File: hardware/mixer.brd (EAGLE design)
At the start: 113.2 x 100 mm, 199 parts, among them IC1 PGA2311, IC10 OPA2134P, IC11 OPA2134P, IC12 OPA2134P, IC13 OPA2134P, IC2 PGA2311, IC3 PGA2311, IC4 PGA2311, IC5 PGA2311, IC6 OPA2134P, IC7 OPA2134P, IC8 OPA2134P, IC9 OPA2134P, Q1 SI2305, Q2 MOSFET-NCHANNEL_SOT23-3, X1 MOLEX_6HORIZONTAL, X2 MOLEX_6HORIZONTAL, X3 MOLEX_4HORIZONTAL, Y1 32768Hz CFPX-217 12.5pF

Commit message: routing
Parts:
- removed C47, C51, C52: 100n, rcl:C0805
- removed C64, C65, C66, C67, C68, C69, C71, C72, C73, C74, C75, C76, C78, C88, C89, C90: 10u, rcl:153CLV-0405
- removed R92, R93, R94, R95: 0R_0805, Simplex-Jumpers:R0805W
- removed U$10, U$3, U$4, U$8: RESETTABLE, Simplex-Fuses:1210
- added C17, C18, C19, C20, C21, C22, C24, C25, C26, C28, C32, C33, C63, C79, C80: 100n, rcl:C0805
- added C92, C96: 10u, rcl:153CLV-0405
- added R96, R97: 0R_0805, Simplex-Jumpers:R0805W
- added R98, R99: DNP, rcl:R0805W
- added U$12, U$13, U$2, U$5, U$6, U$9: RESETTABLE, Simplex-Fuses:1210
- added X4: inputs, con-3m:PAK100/2500-14
- added X5: outputs, con-3m:PAK100/2500-14
- X2: value MOLEX_6HORIZONTAL -> 2514-; device Simplex-Connectors:0530480610 -> con-3m:PAK100/2500-14
- X3: value MOLEX_4HORIZONTAL -> display
- moved C87 813.4 mm to (4.60, 60.5)
- moved C58 769.7 mm to (38.5, 89.5), flipped to the bottom, turned to 270 degrees
- moved C91 767.9 mm to (19.4, 3.60)
- moved C59 753.2 mm to (38.5, 70.5), flipped to the bottom, turned to 270 degrees
- moved C60 737.8 mm to (38.6, 52.2), flipped to the bottom, turned to 270 degrees
- moved C61 722.1 mm to (38.6, 33.6), flipped to the bottom, turned to 270 degrees
- moved C62 705.7 mm to (38.6, 14.2), flipped to the bottom, turned to 270 degrees
- moved LED2 661.9 mm to (12.4, 54.8)
- moved R33 661.9 mm to (23.4, 59.5)
- moved C45 631.9 mm to (22.4, 90.2), turned to 180 degrees
- moved C84 630.1 mm to (10.4, 59.6)
- moved C85 630.1 mm to (14.4, 59.6)
- moved C86 630.1 mm to (6.40, 53.5)
- moved C50 612.5 mm to (22.4, 71.0), turned to 180 degrees
- moved C81 608.1 mm to (22.4, 52.9), turned to 180 degrees
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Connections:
- removed net +3V: C84.1, C85.1, C86.1, C87.+, R95.2
- removed net +5V_DIG: Q1.2, R37.2, R92.1
- removed net A+5V: C29.1, C30.1, C31.1, C34.1, C35.1, C36.1, C37.1, C46.1, C47.1, C48.1, C49.1, C58.2, C59.2, C60.2, C61.2, C62.2, C64.+, C65.+, C66.+, C67.+, C68.+, C69.+, C70.+, IC1.12, IC10.8, IC11.8, IC12.8, IC13.8, IC2.12, IC3.12, IC4.12, IC5.12, IC6.8, IC7.8, IC8.8, IC9.8, R94.1
- removed net A-5V: C38.1, C39.1, C40.1, C41.1, C42.1, C43.1, C44.1, C51.1, C52.1, C53.1, C54.1, C58.1, C59.1, C60.1, C61.1, C62.1, C71.-, C72.-, C73.-, C74.-, C75.-, C76.-, C77.-, IC1.13, IC10.4, IC11.4, IC12.4, IC13.4, IC2.13, IC3.13, IC4.13, IC5.13, IC6.4, IC7.4, IC8.4, IC9.4, R93.1
- removed net N$24: U$4.P$2, X2.4
- removed net N$25: U$8.P$2, X2.3
- removed net N$3: R92.2, U$8.P$1
- removed net N$34: U$10.P$2, X2.2
- removed net N$6: R95.1, U$10.P$1
- removed net N$60: R94.2, U$3.P$1
- removed net N$62: R93.2, U$4.P$1
- removed net N$63: U$3.P$2, X2.5
- removed net VCC: R34.2, U$11.11, U$11.28, U$11.7, X1.4
- new net +15V: C17.1, C18.1, C24.1, C25.1, C33.1, C63.1, C79.1, C80.1, C92.+, IC10.8, IC11.8, IC12.8, IC13.8, U$2.P$2
- new net +5V: C26.2, C28.2, C29.1, C30.1, C31.1, C32.2, C34.1, C35.1, C36.1, C37.1, C46.2, C48.1, C49.1, C58.2, C59.2, C60.2, C61.2, C62.2, C70.+, IC1.12, IC2.12, IC3.12, IC4.12, IC5.12, IC6.8, IC7.8, IC8.8, IC9.8, U$6.P$2
- new net +5V/1: Q1.2, R37.2, U$12.P$2
- new net -15V: C19.1, C20.1, C21.1, C22.1, C33.2, C63.2, C79.2, C80.2, C96.+, IC10.4, IC11.4, IC12.4, IC13.4, U$5.P$2
- new net -5V: C26.1, C28.1, C32.1, C38.1, C39.1, C40.1, C41.1, C42.1, C43.1, C44.1, C46.1, C53.1, C54.1, C58.1, C59.1, C60.1, C61.1, C62.1, C77.-, IC1.13, IC2.13, IC3.13, IC4.13, IC5.13, IC6.4, IC7.4, IC8.4, IC9.4, U$9.P$2
- new net 3V3: C84.1, C85.1, C86.1, C87.+, R34.2, U$11.11, U$11.28, U$11.7, U$13.P$2, X1.4, X3.1
- new net N$79: IC5.9, R97.1, R99.2
- new net N$80: JP2.2, R97.2
- new net N$85: U$2.P$1, X2.12
- new net N$86: U$5.P$1, X2.10
- new net N$88: U$6.P$1, X2.8
- new net N$89: U$9.P$1, X2.6
- new net N$90: U$12.P$1, X2.4
- new net N$91: U$13.P$1, X2.2
- net +5V_PGA: no longer C78.+, C88.+, C89.+, C90.+
- net AGND: now also C17.2, C18.2, C19.2, C20.2, C21.2, C22.2, C24.2, C25.2, C92.-, C96.-, R98.1, R99.1, X2.11, X2.13, X2.7, X2.9, X4.1, X4.10, X4.13, X4.4, X4.7, X5.10, X5.12, X5.14, X5.2, X5.4, X5.6, X5.8; no longer C46.2, C47.2, C51.2, C52.2, C64.-, C65.-, C66.-, C67.-, C68.-, C69.-, C71.+, C72.+, C73.+, C74.+, C75.+, C76.+, X2.6
- net DGND: now also X2.3, X2.5; no longer C78.-, C88.-, C89.-, C90.-, X3.1
- net FRONT_L: now also X4.2
- net FRONT_R: now also X4.3
- net LINE_L: now also X4.5
- net LINE_R: now also X4.6
- net M_FRONT_L: now also X5.11
- net M_FRONT_R: now also X5.13
- net M_REAR_L: now also X5.7
- net M_REAR_R: now also X5.9
- net N$36: now also R96.2; no longer IC5.16
- net N$42: now also IC5.16, R96.1, R98.2; no longer IC5.9, JP2.2
- net REAR_L: now also X4.11
- net REAR_R: now also X4.12
- net SPDIF_L: now also X4.8
- net SPDIF_R: now also X4.9
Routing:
- net +5V: track 0.00 -> 259.3 mm, vias 0 -> 9
- net -5V: track 0.00 -> 256.0 mm, vias 0 -> 16
- net +5V_PGA: track 0.00 -> 135.9 mm, vias 0 -> 5
- net AGND: track 26.3 -> 148.1 mm, vias 13 -> 53
- net +15V: track 0.00 -> 102.7 mm, vias 0 -> 4
- net -15V: track 0.00 -> 101.7 mm, vias 0 -> 4
- net CLK: track 0.00 -> 90.7 mm
- net MOSI: track 0.00 -> 90.6 mm, vias 0 -> 5
- net DGND: track 0.00 -> 41.9 mm, vias 0 -> 5
- net N$34: track 5.36 -> 0.00 mm
- net N$63: track 5.18 -> 0.00 mm
- net N$20: track 4.18 -> 9.03 mm
- net N$25: track 4.49 -> 0.00 mm
- net N$24: track 4.45 -> 0.00 mm
- net N$43: track 0.00 -> 3.57 mm
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
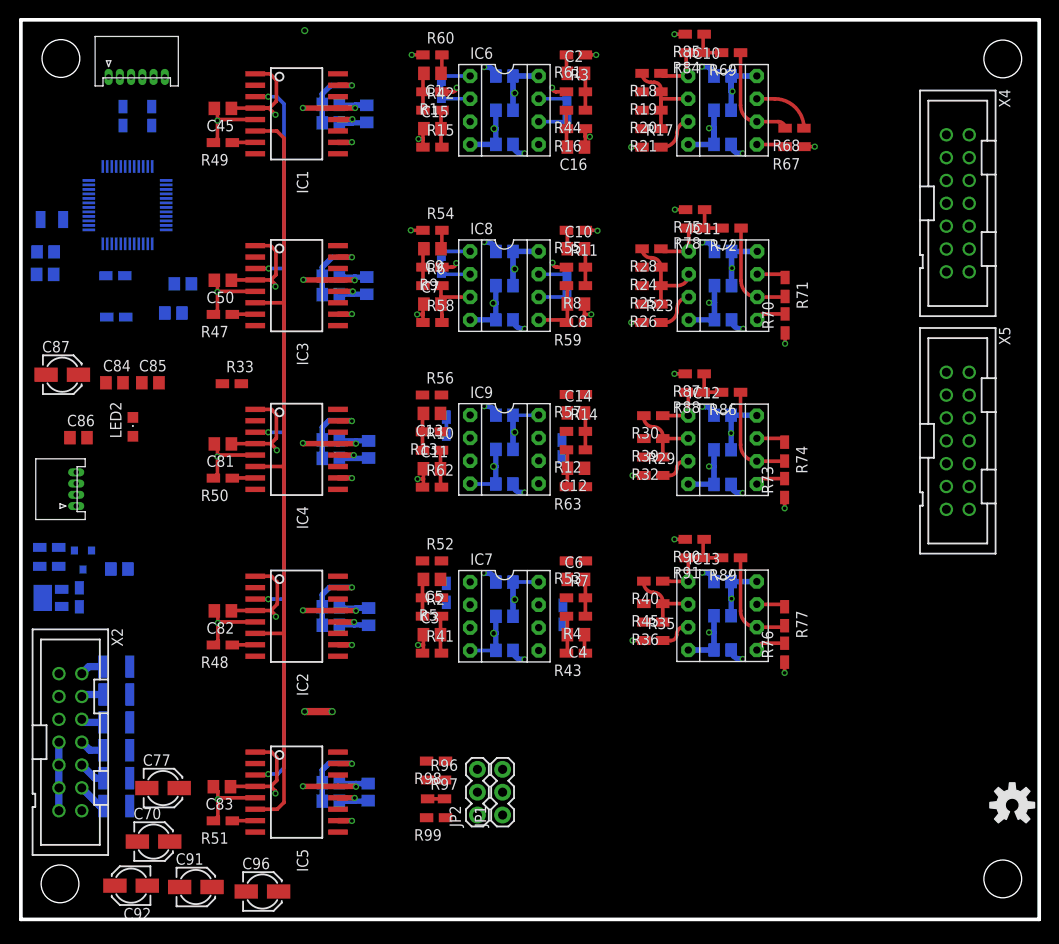
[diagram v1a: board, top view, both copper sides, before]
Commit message: routing
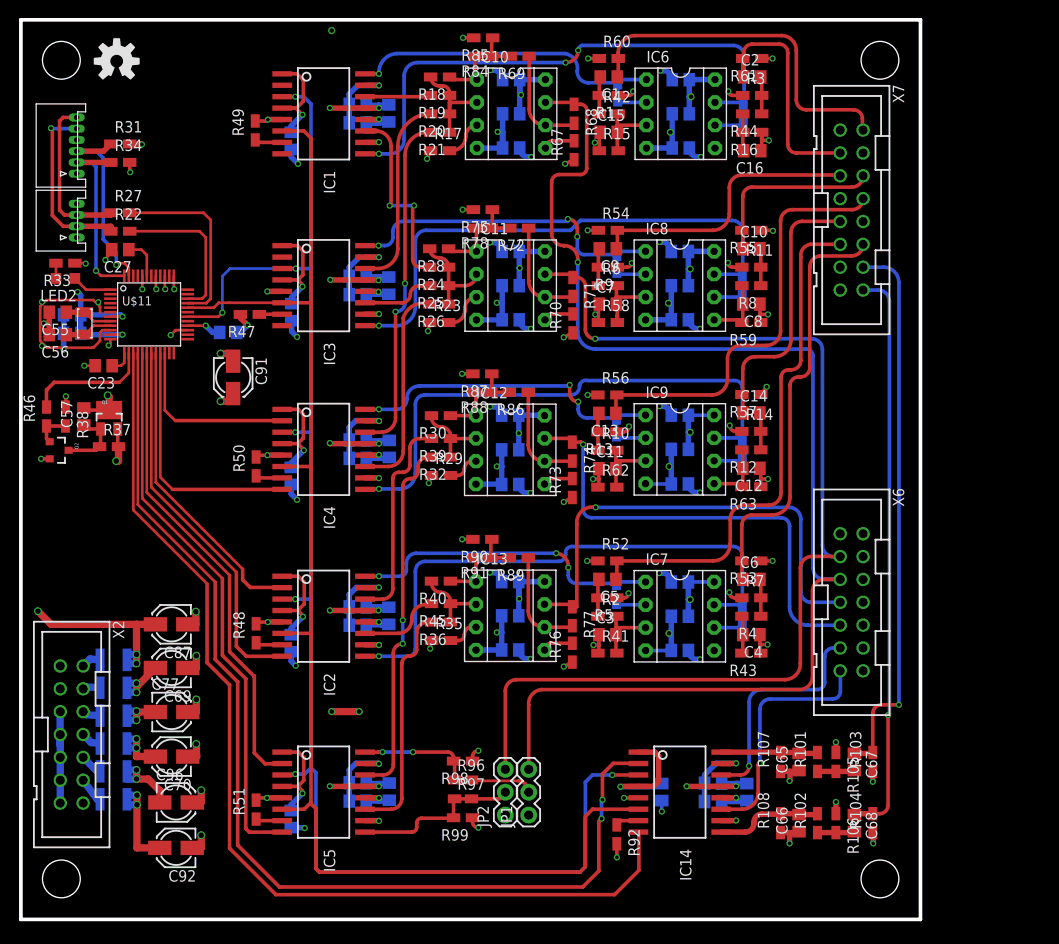
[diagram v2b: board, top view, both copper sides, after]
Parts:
- removed X4: inputs, con-3m:PAK100/2500-14
- removed X5: outputs, con-3m:PAK100/2500-14
- added C47, C51, C52, C64: 100n, rcl:C0805
- added C65, C66: 1n, rcl:C0805
- added C67, C68: 1u, rcl:C0805
- added C69: 10u, rcl:153CLV-0405
- added IC14: PGA2311, Simplex-ICs:SO-16
- added R101, R102: 1K, rcl:R0805W
- added R103, R104, R107, R108: DNP, rcl:R0805W
- added R105, R106: 100K, rcl:R0805W
- added R92: 47K, rcl:R0805W
- added X6: 2514-, con-3m:PAK100/2500-14
- added X7: 2516-, con-3m:PAK100/2500-16
- moved U$7 129.4 mm to (10.7, 95.4)
- moved C91 56.8 mm to (23.6, 60.2), turned to 270 degrees
- moved C87 30.3 mm to (16.8, 32.8), turned to 180 degrees
- moved X3 29.9 mm to (6.20, 75.8)
- moved R68 24.6 mm to (61.5, 89.5), turned to 270 degrees
- moved R67 24.5 mm to (61.5, 85.5), turned to 90 degrees
- moved R73 23.6 mm to (61.3, 48.0)
- moved R74 23.6 mm to (61.3, 52.0)
- moved R76 23.6 mm to (61.3, 29.6)
- moved R77 23.6 mm to (61.3, 33.7)
- moved R87 23.6 mm to (51.3, 60.6)
- moved R88 23.6 mm to (51.3, 58.6)
- moved R90 23.6 mm to (51.3, 42.2)
- moved R91 23.6 mm to (51.3, 40.2)
- moved C17 23.6 mm to (54.4, 37.5)
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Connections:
- net V_REAR_PAN_L renamed V_CENTER
- net V_REAR_PAN_R renamed V_SW
- removed net N$39: LED2.A, U$11.22
- new net CENTER: C67.1, R103.2, X7.14
- new net CS6: IC14.2, U$11.16
- new net M6: IC14.8, U$11.15
- new net M_CENTER: IC14.14, X6.11
- new net M_SW: IC14.11, X6.13
- new net N$24: C65.2, IC14.16, R101.2, R107.2
- new net N$3: IC14.7, R92.1
- new net N$34: C66.2, IC14.9, R102.2, R108.2
- new net N$6: LED2.A, U$11.1
- new net N$62: C67.2, R101.1, R105.2
- new net N$63: C68.2, R102.1, R106.2
- new net SW: C68.1, R104.2, X7.16
- net +5V: now also C51.2, C52.1, IC14.12
- net +5V/1: now also C69.+
- net +5V_PGA: now also C47.1, IC14.1, IC14.4
- net -15V: now also C96.-; no longer C96.+
- net -5V: now also C51.1, C64.1, IC14.13
- net AGND: now also C52.2, C64.2, C65.1, C66.1, C96.+, IC14.10, IC14.15, R103.1, R104.1, R105.1, R106.1, R107.1, R108.1, X2.5, X6.10, X6.12, X6.14, X6.2, X6.4, X6.6, X6.8, X7.1, X7.10, X7.13, X7.15, X7.4, X7.7; no longer C96.-, X4.1, X4.10, X4.13, X4.4, X4.7, X5.10, X5.12, X5.14, X5.2, X5.4, X5.6, X5.8
- net CLK: now also IC14.6, U$11.32
- net CS2: now also U$11.20
- net CS4: now also U$11.22
- net CS5: now also U$11.18
- net DGND: now also C47.2, C69.-, IC14.5, R92.2; no longer X2.5
- net FRONT_L: now also X7.2; no longer X4.2
- net FRONT_R: now also X7.3; no longer X4.3
- net LINE_L: now also X7.5; no longer X4.5
- net LINE_R: now also X7.6; no longer X4.6
- net M2: now also U$11.19
- net M4: now also U$11.21
- net M5: now also U$11.17
- net MOSI: now also IC14.3, U$11.30
- net M_FRONT_L: now also X6.5; no longer X5.11
- net M_FRONT_R: now also X6.3; no longer X5.13
- net M_REAR_L: now also X6.9; no longer X5.7
- net M_REAR_R: now also X6.7; no longer X5.9
- net PGA_EN: now also U$11.14
- net REAR_L: now also X7.11; no longer X4.11
- net REAR_R: now also X7.12; no longer X4.12
- net SPDIF_L: now also X7.8; no longer X4.8
- net SPDIF_R: now also X7.9; no longer X4.9
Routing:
- net M_FRONT_L: track 6.60 -> 153.6 mm, vias 0 -> 1
- net 3V3: track 0.00 -> 131.8 mm, vias 0 -> 8
- net M_FRONT_R: track 3.23 -> 126.1 mm, vias 0 -> 1
- net CS6: track 0.00 -> 117.5 mm, vias 0 -> 2
- net M6: track 0.00 -> 112.5 mm
- net AGND: track 148.1 -> 252.6 mm, vias 53 -> 77
- net +5V_PGA: track 135.9 -> 231.6 mm, vias 5 -> 8
- net MOSI: track 90.6 -> 164.6 mm, vias 5 -> 7
- net SW: track 0.00 -> 63.8 mm, vias 0 -> 1
- net M5: track 0.00 -> 61.9 mm
- net N$7: track 0.00 -> 61.5 mm, vias 0 -> 1
- net CENTER: track 0.00 -> 61.4 mm, vias 0 -> 1
- net N$26: track 0.00 -> 61.0 mm, vias 0 -> 1
- net CLK: track 90.7 -> 151.2 mm
- net REAR_L: track 0.00 -> 57.5 mm
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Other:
- board size 113.2 x 100 mm -> 100 x 100 mm
